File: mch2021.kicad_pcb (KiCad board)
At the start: 4 copper layers, 100 x 100 mm, 162 parts, among them J1 USB_C_Receptacle_USB2.0, J2 SAO, J3 AudioJack3, J4 SAO, J5 Micro SD card, J6 PMOD, J7 LCD, J8 GPIO, Q1 Q_PMOS_GSD, Q2 Q_NMOS_GSD, Q3 Q_NMOS_GSD, SW1 Power switch, SW2 Start, SW3 Select, SW4 Menu, SW5 Home, SW6 Back, SW7 Accept, U1 SY8079AAC, U10 74LVC1G125, U11 STM32F103C8Tx, U12 PCA9555PW, U13 ESP32-WROVER, U2 SY8079AAC, U3 XT4054K421MR-G, U4 SY6280AAC, U5 SY6280AAC, U6 MPU-6050, U7 74LVC1G125, U8 ICE40UP5K-SG48ITR, U9 LY68L6400, Y1 16MHz

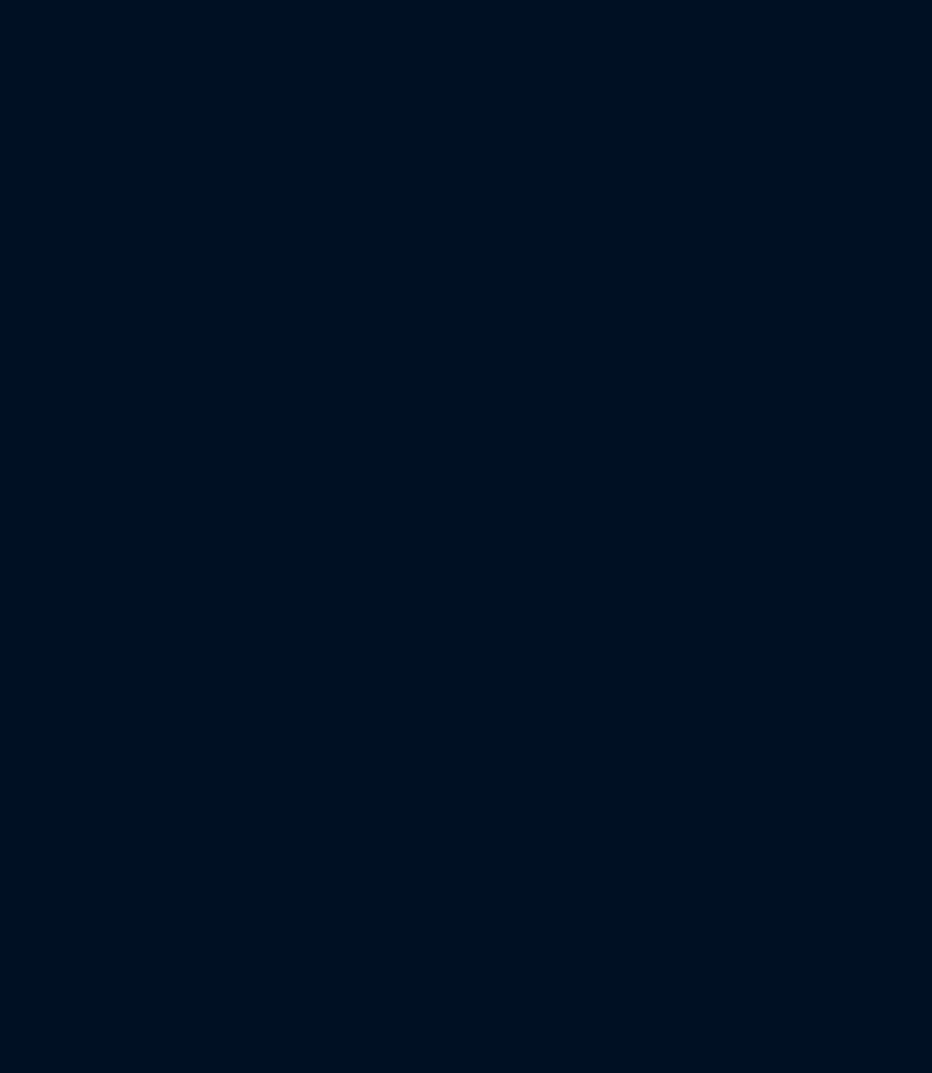
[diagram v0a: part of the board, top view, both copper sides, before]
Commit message: More work on prototype 2
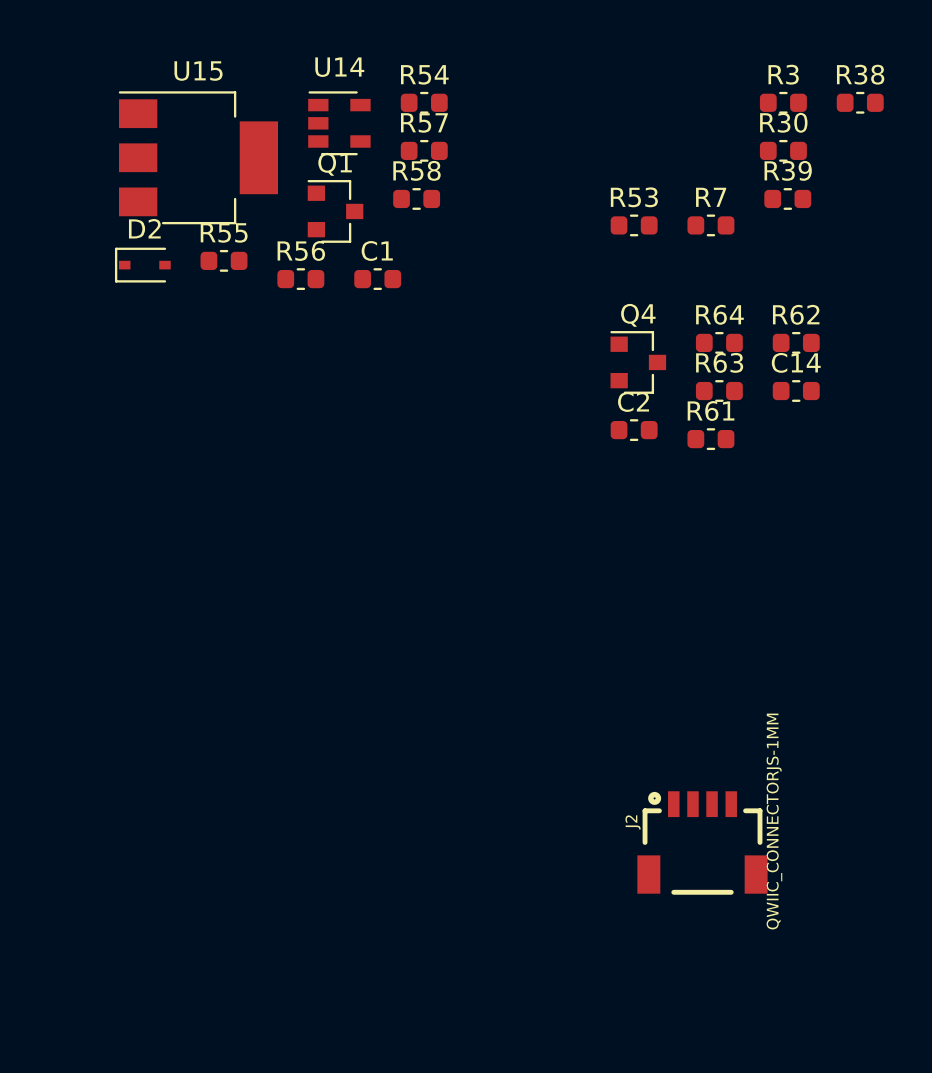
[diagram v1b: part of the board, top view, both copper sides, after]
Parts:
- added C1: 100n, Capacitor_SMD:C_0603_1608Metric, F.Cu at (137.3, 11.2)
- added C14: 22p, Capacitor_SMD:C_0603_1608Metric, F.Cu at (159.1, 17.1)
- added C2: 22p, Capacitor_SMD:C_0603_1608Metric, F.Cu at (150.7, 19.1)
- added D2: NSVR0320MW2T1G, Diode_SMD:D_SOD-323, F.Cu at (125.1, 10.5)
- added J2: QWIIC_CONNECTORJS-1MM, Connectors:1X04_1MM_RA, F.Cu at (154.2, 38.6)
- added Q1: Q_NMOS_GSD, Package_TO_SOT_SMD:SOT-23, F.Cu at (135.1, 7.70)
- added Q4: Q_NMOS_GSD, Package_TO_SOT_SMD:SOT-23, F.Cu at (150.9, 15.6)
- added R3: 10k, Resistor_SMD:R_0603_1608Metric, F.Cu at (158.4, 2.03)
- added R30: 10k, Resistor_SMD:R_0603_1608Metric, F.Cu at (158.4, 4.54)
- added R38: 10k, Resistor_SMD:R_0603_1608Metric, F.Cu at (162.5, 2.03)
- added R39: 10k, Resistor_SMD:R_0603_1608Metric, F.Cu at (158.7, 7.05)
- added R53: 10k, Resistor_SMD:R_0603_1608Metric, F.Cu at (150.7, 8.43)
- added R54: 10k, Resistor_SMD:R_0603_1608Metric, F.Cu at (139.7, 2.03)
- added R55: 10k, Resistor_SMD:R_0603_1608Metric, F.Cu at (129.3, 10.3)
- added R56: 10k, Resistor_SMD:R_0603_1608Metric, F.Cu at (133.3, 11.2)
- added R57: 100k, Resistor_SMD:R_0603_1608Metric, F.Cu at (139.7, 4.54)
- added R58: 10k, Resistor_SMD:R_0603_1608Metric, F.Cu at (139.3, 7.05)
- added R61: 47, Resistor_SMD:R_0603_1608Metric, F.Cu at (154.7, 19.6)
- added R62: 47, Resistor_SMD:R_0603_1608Metric, F.Cu at (159.1, 14.6)
- added R63: 10k, Resistor_SMD:R_0603_1608Metric, F.Cu at (155.1, 17.1)
- added R64: 10k, Resistor_SMD:R_0603_1608Metric, F.Cu at (155.1, 14.6)
- added R7: 10k, Resistor_SMD:R_0603_1608Metric, F.Cu at (154.7, 8.43)
- added U14: SY6280AAC, Package_TO_SOT_SMD:SOT-23-5, F.Cu at (135.3, 3.10)
- added U15: AMS1117-3.3, Package_TO_SOT_SMD:SOT-223-3_TabPin2, F.Cu at (127.9, 4.90)
- R43: value 10k -> DNP
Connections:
- C1 pad 2: Net-(C1-Pad2) -> (no net)
- D10 pad 3: (no net) -> /CC1
- J1 pad A8: SBU1 -> (no net)
- J1 pad B8: SBU2 -> (no net)
- J2 pad 5: /STM32/SAO_IO2 -> (no net)
- J2 pad 6: /STM32/SAO_IO3 -> (no net)
- J3 pad R: Net-(C2-Pad1) -> (no net)
- J3 pad T: Net-(C1-Pad2) -> (no net)
- J5 pad 1: SD_D2 -> Net-(J5-Pad1)
- J5 pad 2: /ESP32/SD_D3 -> Net-(J5-Pad2)
- J5 pad 3: SD_CMD -> /ESP32/SD_CMD
- J5 pad 7: SD_D0 -> /ESP32/SD_D0
- J5 pad 8: /ESP32/SD_D1 -> Net-(J5-Pad8)
- J8 pad 2: Net-(J8-Pad2) -> (no net)
- J8 pad 3: Net-(J8-Pad3) -> (no net)
- LS1 pad 2: SPK -> (no net)
- R10 pad 1: /BUTTONS/CHARGING -> /POWER/CHARGING
- R11 pad 2: /ESP32/PWR_SDCARD_ENABLE -> /POWER/PWR_SDCARD_ENABLE
- R38 pad 2: Net-(R38-Pad2) -> (no net)
- R39 pad 2: Net-(R39-Pad2) -> (no net)
- R46 pad 1: SD_D0 -> /ESP32/SD_D0
- R49 pad 2: SD_D2 -> Net-(R49-Pad2)
- R50 pad 1: SD_D2 -> Net-(R49-Pad2)
- R54 pad 2: SD_CMD -> (no net)
- R55 pad 2: SD_D0 -> (no net)
- R56 pad 2: /ESP32/SD_D1 -> (no net)
- R57 pad 2: SD_D2 -> (no net)
- R58 pad 2: /ESP32/SD_D3 -> (no net)
- R59 pad 2: SD_CMD -> /ESP32/SD_CMD
- R60 pad 1: SD_CMD -> /ESP32/SD_CMD
- R61 pad 1: SBU1 -> (no net)
- R62 pad 2: SBU2 -> (no net)
- RN1 pad 5: ESP32_AUDIO_R -> (no net)
- RN1 pad 7: ESP32_AUDIO_L -> (no net)
- SW1 pad 1: Net-(D2-Pad1) -> Net-(R55-Pad1)
- SW1 pad 2: VIN -> VBAT
- SW1 pad 3: VUSB -> (no net)
- U11 pad 1: +3V3 -> BAT_3.3
- U11 pad 12: /ESP32/ESP32_RX -> /STM32/FPGA_RX
- U11 pad 13: /ESP32/ESP32_TX -> /STM32/FPGA_TX
- U11 pad 18: /STM32/SAO_IO3 -> /ESP32/ESP32_EN
- U11 pad 19: /STM32/SAO_IO2 -> Net-(R62-Pad2)
- U11 pad 2: /ESP32/ESP32_EN -> Net-(Q4-Pad3)
- U11 pad 20: /STM32/SAO_IO1 -> /POWER/CHARGING
- U11 pad 21: /STM32/SAO_IO0 -> /ACCELEROMETER/I2C_SCL
- U11 pad 22: Net-(U10-Pad2) -> /ACCELEROMETER/I2C_SDA
- U11 pad 25: Net-(J8-Pad3) -> /STM32/SAO_IO0
- U11 pad 26: Net-(J8-Pad2) -> /STM32/SAO_IO1
- U11 pad 28: Net-(U10-Pad2) -> /POWER/PWR_SDCARD_ENABLE
- U11 pad 3: /ESP32/ESP32_BL -> Net-(C14-Pad1)
- U11 pad 30: /STM32/FPGA_RX -> /ESP32/ESP32_RX
- U11 pad 31: /STM32/FPGA_TX -> /ESP32/ESP32_TX
- U11 pad 38: SPK -> Net-(R64-Pad2)
- U11 pad 4: (no net) -> Net-(C2-Pad1)
- U11 pad 42: /ACCELEROMETER/I2C_SCL -> Net-(U10-Pad2)
- U11 pad 43: /ACCELEROMETER/I2C_SDA -> (no net)
- U11 pad 45: /FPGA/LCD_ENABLE -> (no net)
- U12 pad 8: /BUTTONS/CHARGING -> (no net)
- U13 pad 10: ESP32_AUDIO_L -> (no net)
- U13 pad 11: ESP32_AUDIO_R -> (no net)
- U13 pad 14: SD_D2 -> Net-(R49-Pad2)
- U13 pad 16: /ESP32/SD_D3 -> (no net)
- U13 pad 23: SD_CMD -> /ESP32/SD_CMD
- U13 pad 24: SD_D0 -> /ESP32/SD_D0
- U13 pad 26: /ESP32/SD_D1 -> (no net)
- U13 pad 29: /ESP32/PWR_SDCARD_ENABLE -> (no net)
- U3 pad 1: /BUTTONS/CHARGING -> /POWER/CHARGING
- U4 pad 4: /ESP32/PWR_SDCARD_ENABLE -> /POWER/PWR_SDCARD_ENABLE
- U7 pad 1: /STM32/LCD_MODE -> /LCD/LCD_IM0
- U8 pad 38: /FPGA/LCD_ENABLE -> (no net)
- U8 pad 42: Net-(R39-Pad2) -> (no net)
- U8 pad 43: Net-(R38-Pad2) -> (no net)
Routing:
- net (no net): track 3.18 -> 376.4 mm, vias 0 -> 10
- net /FPGA/LCD_ENABLE: track 80.2 -> 0.00 mm
- net ESP32_AUDIO_L: track 68.2 -> 0.00 mm, vias 2 -> 0
- net ESP32_AUDIO_R: track 65.4 -> 0.00 mm, vias 2 -> 0
- net Net-(R39-Pad2): track 65.4 -> 0.00 mm, vias 2 -> 0
- net Net-(R38-Pad2): track 61.6 -> 0.00 mm, vias 2 -> 0
- net SBU1: track 13.2 -> 0.00 mm, vias 2 -> 0
- net Net-(C1-Pad2): track 9.73 -> 0.00 mm
- net SBU2: track 9.47 -> 0.00 mm
